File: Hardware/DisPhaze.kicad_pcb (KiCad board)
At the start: 2 copper layers, 71 x 24.1 mm, 13 parts, among them J1 Conn_01x27, J2 Conn_01x27, J3 Conn_01x04_Male, U1 STM32F405RGTx, Y1 Crystal

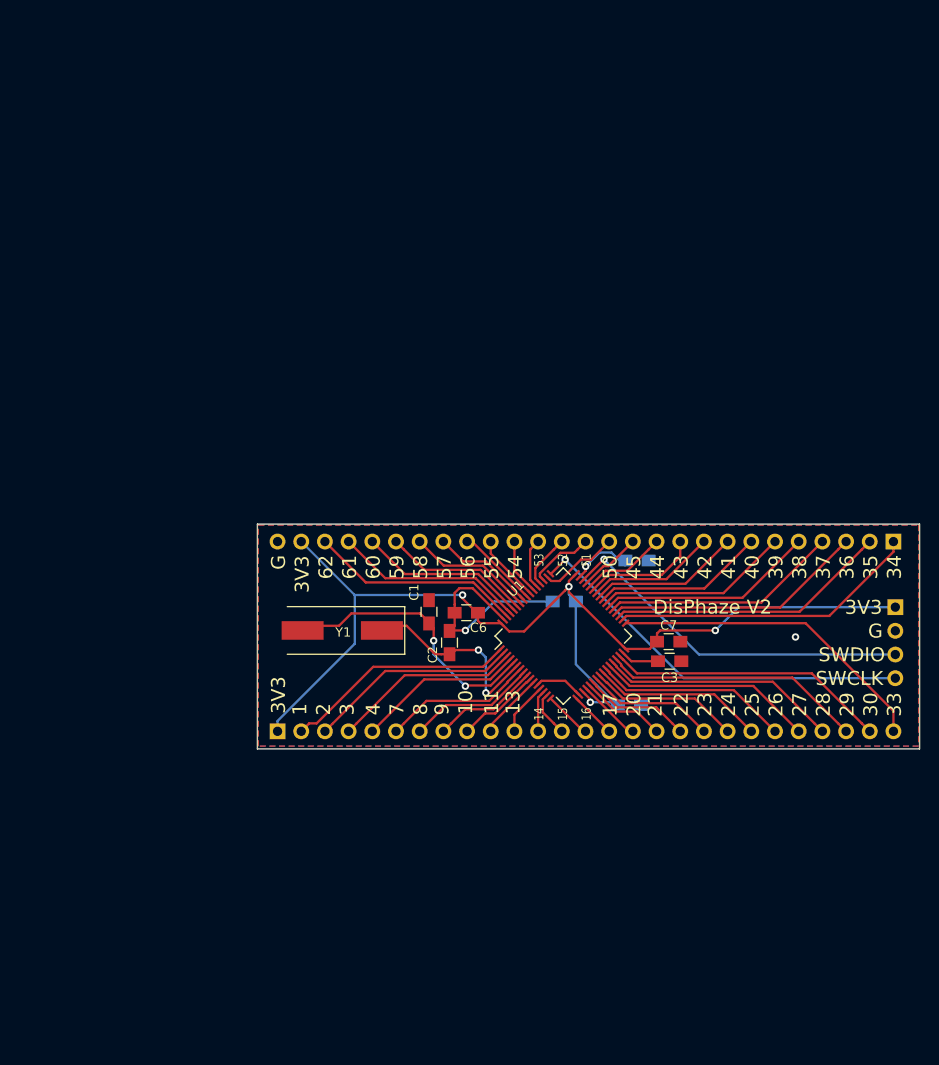
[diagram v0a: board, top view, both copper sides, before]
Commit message: Start PCB layout
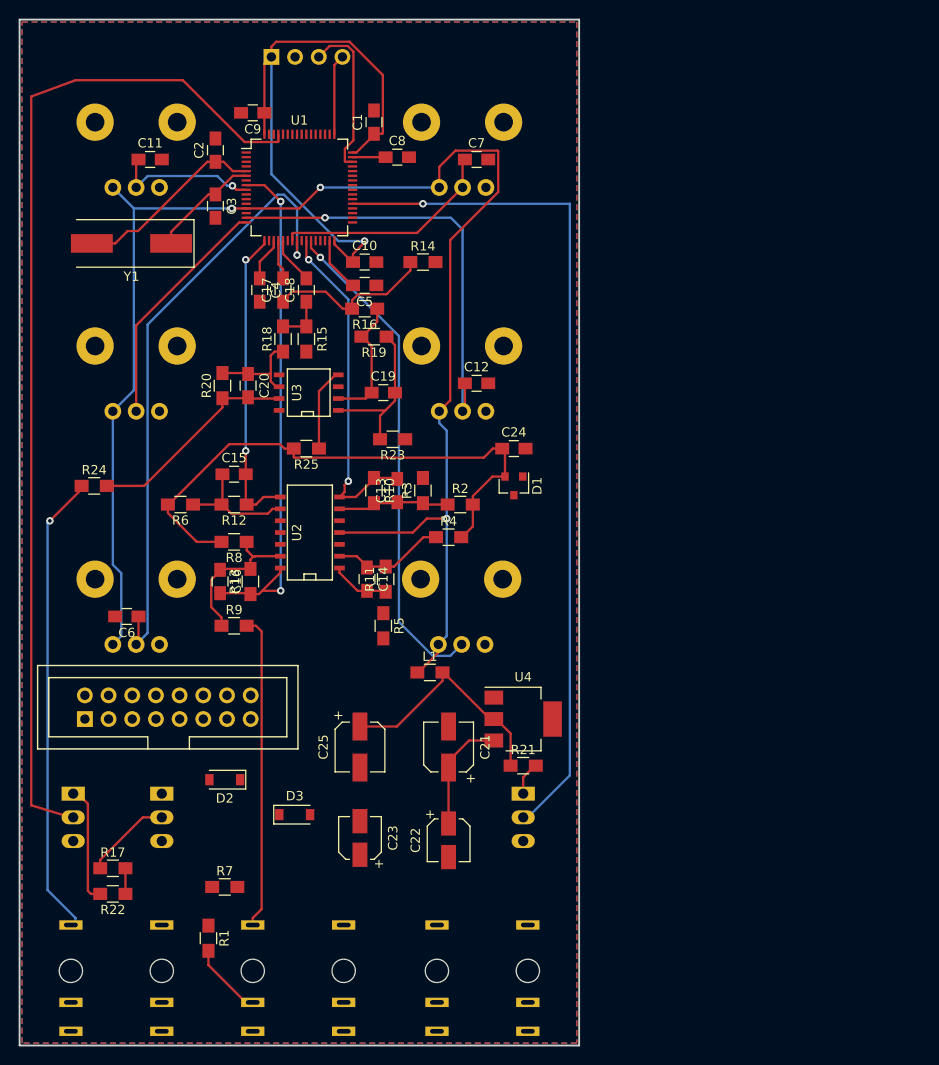
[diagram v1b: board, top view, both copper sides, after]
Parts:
- added C10: 100nF, Capacitors_SMD:C_0805_HandSoldering, F.Cu at (137.0, 76.0)
- added C11: 100nF, Capacitors_SMD:C_0805_HandSoldering, F.Cu at (114.0, 65.0)
- added C12: 100nF, Capacitors_SMD:C_0805_HandSoldering, F.Cu at (149.0, 89.0)
- added C13: 1nF, Capacitors_SMD:C_0805_HandSoldering, F.Cu at (140.5, 100.5)
- added C14: 2.2nF, Capacitors_SMD:C_0805_HandSoldering, F.Cu at (137.2, 110.0)
- added C15: 2.2nF, Capacitors_SMD:C_0805_HandSoldering, F.Cu at (123.0, 98.8)
- added C16: 1nF, Capacitors_SMD:C_0805_HandSoldering, F.Cu at (121.5, 110.2)
- added C17: 10uF, Capacitors_SMD:C_0805_HandSoldering, F.Cu at (128.2, 79.0)
- added C18: 10uF, Capacitors_SMD:C_0805_HandSoldering, F.Cu at (130.8, 79.0)
- added C19: 18pF, Capacitors_SMD:C_0805_HandSoldering, F.Cu at (139.0, 90.0)
- added C20: 18pF, Capacitors_SMD:C_0805_HandSoldering, F.Cu at (124.5, 89.2)
- added C21: 47uF, Capacitors_SMD:CP_Elec_5x5.8, F.Cu at (146.0, 128.0)
- added C22: 22uF, Capacitors_SMD:CP_Elec_4x5.8, F.Cu at (146.0, 138.0)
- added C23: 22uF, Capacitors_SMD:CP_Elec_4x5.8, F.Cu at (136.5, 137.8)
- added C24: 100nF, Capacitors_SMD:C_0805_HandSoldering, F.Cu at (153.0, 96.0)
- added C25: 47uF, Capacitors_SMD:CP_Elec_5x5.8, F.Cu at (136.5, 128.0)
- added C9: 100nF, Capacitors_SMD:C_0805_HandSoldering, F.Cu at (125.0, 60.0)
- added CTune1: B10k, Potentiometers:Potentiometer_Alps_RK09K_Horizontal, B.Cu at (144.9, 117.0)
- added D1: LM4040DBZ-5, TO_SOT_Packages_SMD:SOT-23, F.Cu at (153.0, 100.0)
- added D2: 1N5819, Diodes_SMD:D_SOD-123, F.Cu at (122.0, 131.5)
- added D3: 1N5819, Diodes_SMD:D_SOD-123, F.Cu at (129.5, 135.2)
- added FTune1: B10k, Potentiometers:Potentiometer_Alps_RK09K_Horizontal, B.Cu at (110.0, 117.0)
- added J4: PD2_Amt_In, Custom_Footprints:THONKICONN_hole, B.Cu at (115.2, 152.0)
- added J5: VCA_In, Custom_Footprints:THONKICONN_hole, B.Cu at (125.0, 152.0)
- added J6: DAC1_Out, Custom_Footprints:THONKICONN_hole, B.Cu at (154.5, 152.0)
- added J7: DAC2_Out, Custom_Footprints:THONKICONN_hole, B.Cu at (105.5, 152.0)
- added J8: Eurorack_16_pin_power, Custom_Footprints:Eurorack_16_pin_header, F.Cu at (107.0, 125.0)
- added L1: L, Resistors_SMD:R_0805_HandSoldering, F.Cu at (144.0, 120.0)
- added PD1Amt1: B10k, Potentiometers:Potentiometer_Alps_RK09K_Horizontal, B.Cu at (145.0, 68.0)
- added PD1Type1: B10k, Potentiometers:Potentiometer_Alps_RK09K_Horizontal, B.Cu at (145.0, 92.0)
- added PD2Amt1: B10k, Potentiometers:Potentiometer_Alps_RK09K_Horizontal, B.Cu at (110.0, 68.0)
- added PD2Type1: B10k, Potentiometers:Potentiometer_Alps_RK09K_Horizontal, B.Cu at (110.0, 92.0)
- added R1: 47k, Resistors_SMD:R_0805_HandSoldering, F.Cu at (120.2, 148.5)
- added R10: 47k, Resistors_SMD:R_0805_HandSoldering, F.Cu at (138.0, 100.5)
- added R11: 56k, Resistors_SMD:R_0805_HandSoldering, F.Cu at (139.2, 110.0)
- added R12: 47k, Resistors_SMD:R_0805_HandSoldering, F.Cu at (123.0, 102.0)
- added R13: 47k, Resistors_SMD:R_0805_HandSoldering, F.Cu at (124.8, 110.2)
- added R14: 47k, Resistors_SMD:R_0805_HandSoldering, F.Cu at (143.2, 76.0)
- added R15: 47k, Resistors_SMD:R_0805_HandSoldering, F.Cu at (130.8, 84.2)
- added R16: 6.3k, Resistors_SMD:R_0805_HandSoldering, F.Cu at (137.0, 81.0)
- added R17: 680R, Resistors_SMD:R_0805_HandSoldering, F.Cu at (110.0, 141.0)
- added R18: 6.3k, Resistors_SMD:R_0805_HandSoldering, F.Cu at (128.2, 84.2)
- added R19: 68k, Resistors_SMD:R_0805_HandSoldering, F.Cu at (138.0, 84.0)
- added R2: 82k, Resistors_SMD:R_0805_HandSoldering, F.Cu at (147.2, 102.0)
- added R20: 68k, Resistors_SMD:R_0805_HandSoldering, F.Cu at (121.8, 89.2)
- added R21: 680R, Resistors_SMD:R_0805_HandSoldering, F.Cu at (154.0, 130.0)
- added R22: 680R, Resistors_SMD:R_0805_HandSoldering, F.Cu at (110.0, 143.8)
- added R23: 1k, Resistors_SMD:R_0805_HandSoldering, F.Cu at (140.0, 95.0)
- added R24: 1k, Resistors_SMD:R_0805_HandSoldering, F.Cu at (108.0, 100.0)
- added R25: 2.2k, Resistors_SMD:R_0805_HandSoldering, F.Cu at (130.8, 96.0)
- added R3: 100k, Resistors_SMD:R_0805_HandSoldering, F.Cu at (143.2, 100.5)
- added R4: 91k, Resistors_SMD:R_0805_HandSoldering, F.Cu at (146.0, 105.5)
- added R5: 100k, Resistors_SMD:R_0805_HandSoldering, F.Cu at (139.0, 115.0)
- added R6: 68k, Resistors_SMD:R_0805_HandSoldering, F.Cu at (117.2, 102.0)
- added R7: 100k, Resistors_SMD:R_0805_HandSoldering, F.Cu at (122.0, 143.0)
- added R8: 68k, Resistors_SMD:R_0805_HandSoldering, F.Cu at (123.0, 106.0)
- added R9: 100k, Resistors_SMD:R_0805_HandSoldering, F.Cu at (123.0, 115.0)
- added SW1: DAC1_RingMod_Switch, Custom_Footprints:SPDTSubMiniature, B.Cu at (154.0, 133.0)
- added SW2: DAC2_Mix_Switch, Custom_Footprints:SPDTSubMiniature, B.Cu at (105.8, 133.0)
- added SW3: Octave_Switch, Custom_Footprints:SPDTSubMiniature, B.Cu at (115.2, 133.0)
- added U2: MCP6004, SMD_Packages:SOIC-14_N, F.Cu at (131.0, 105.0)
- added U3: TL072, SMD_Packages:SOIC-8-N, F.Cu at (131.0, 90.0)
- added U4: LM1117-3.3, TO_SOT_Packages_SMD:SOT-223, F.Cu at (154.0, 125.0)
- C1: value 18pF -> 100nF
- C3: value 2.2uF -> 18pF
- C4: value 2.2uF -> 100nF; moved to F.Cu
- C5, C8: value 100nF -> 2.2uF; moved to F.Cu
- J1: value Conn_01x27 -> SWD_Header; footprint Custom_Footprints:Connector_27x2.54mm -> Custom_Footprints:4pin_header
- J2: value Conn_01x27 -> PItch_In; footprint Custom_Footprints:Connector_27x2.54mm -> Custom_Footprints:THONKICONN_hole; moved to B.Cu
- J3: value Conn_01x04_Male -> PD1_Amt_In; footprint Custom_Footprints:4pin_header -> Custom_Footprints:THONKICONN_hole; moved to B.Cu
- moved J2 74.8 mm to (134.8, 152.0)
- moved J1 72.3 mm to (127.0, 54.0)
- moved C3 68.9 mm to (121.0, 70.0), turned to 270 degrees
- moved C8 63.8 mm to (140.5, 64.8)
- moved J3 62.7 mm to (144.8, 152.0), turned to 180 degrees
- moved C2 58.5 mm to (121.0, 64.0)
- moved U1 55.8 mm to (130.0, 68.0), turned to 0 degrees
- moved C7 55.7 mm to (149.0, 65.0)
- moved C1 52.8 mm to (138.0, 61.0)
- moved C4 49.8 mm to (125.8, 79.0), turned to 270 degrees
- moved Y1 47.3 mm to (112.0, 74.0)
- moved C5 40.1 mm to (137.0, 78.5)
- moved C6 36.4 mm to (111.5, 114.0)
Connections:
- C1 pad 1: Net-(C1-Pad1) -> +3V3
- C3 pad 1: GND -> Net-(C3-Pad1)
- C3 pad 2: Net-(C3-Pad2) -> GND
- C4 pad 1: Net-(C4-Pad1) -> +3V3
- C5 pad 1: +3V3 -> GND
- C5 pad 2: GND -> Net-(C5-Pad2)
- C6 pad 1: +3V3 -> FTUNE
- C7 pad 1: +3V3 -> PD1_POT
- C8 pad 1: +3V3 -> Net-(C8-Pad1)
- J1 pad 2: p1 -> GND
- J1 pad 3: p2 -> SWDIO
- J1 pad 4: p3 -> SWCLK
- J2 pad 1: p34 -> GND
- J2 pad 2: p35 -> CV_IN
- J2 pad 3: p36 -> Net-(J2-Pad3)
- J3 pad 1: +3V3 -> GND
- J3 pad 3: SWDIO -> Net-(J3-Pad3)
- U1 pad 1: p1 -> Net-(U1-Pad1)
- U1 pad 10: p10 -> PD1_CV
- U1 pad 11: p11 -> Net-(U1-Pad11)
- U1 pad 13: p13 -> +3.3VA
- U1 pad 14: p14 -> Net-(U1-Pad14)
- U1 pad 15: p15 -> PD1_TYPE
- U1 pad 16: p16 -> PD2_TYPE
- U1 pad 17: p17 -> PD2_CV
- U1 pad 2: p2 -> Net-(U1-Pad2)
- U1 pad 20: p20 -> DAC1_OUT
- U1 pad 21: p21 -> DAC2_OUT
- U1 pad 22: p22 -> Net-(U1-Pad22)
- U1 pad 23: p23 -> PD1_POT
- U1 pad 24: p24 -> FTUNE
- U1 pad 25: p25 -> Net-(U1-Pad25)
- U1 pad 26: p26 -> V_OCT_CV
- U1 pad 27: p27 -> CTUNE
- U1 pad 28: p28 -> Net-(U1-Pad28)
- U1 pad 29: p29 -> Net-(U1-Pad29)
- U1 pad 3: p3 -> Net-(U1-Pad3)
- U1 pad 30: p30 -> Net-(U1-Pad30)
- U1 pad 31: Net-(C3-Pad2) -> Net-(C5-Pad2)
- U1 pad 33: p33 -> OCTAVE_UP
- U1 pad 34: p34 -> OCTAVE_DN
- U1 pad 35: p35 -> Net-(U1-Pad35)
- U1 pad 36: p36 -> Net-(U1-Pad36)
- U1 pad 37: p37 -> DAC1_RING_MOD
- U1 pad 38: p38 -> Net-(U1-Pad38)
- U1 pad 39: p39 -> Net-(U1-Pad39)
- U1 pad 4: p4 -> Net-(U1-Pad4)
- U1 pad 40: p40 -> Net-(U1-Pad40)
- U1 pad 41: p41 -> Net-(U1-Pad41)
- U1 pad 42: p42 -> Net-(U1-Pad42)
- U1 pad 43: p43 -> Net-(U1-Pad43)
- U1 pad 44: p44 -> Net-(U1-Pad44)
- U1 pad 45: p45 -> Net-(U1-Pad45)
- U1 pad 47: Net-(C4-Pad1) -> Net-(C8-Pad1)
- U1 pad 5: Net-(C1-Pad1) -> Net-(C2-Pad1)
- U1 pad 50: p50 -> Net-(U1-Pad50)
- U1 pad 51: p51 -> Net-(U1-Pad51)
- U1 pad 52: p52 -> Net-(U1-Pad52)
- U1 pad 53: p53 -> Net-(U1-Pad53)
- U1 pad 54: p54 -> Net-(U1-Pad54)
- U1 pad 55: p55 -> Net-(U1-Pad55)
- U1 pad 56: p56 -> Net-(U1-Pad56)
- U1 pad 57: p57 -> Net-(U1-Pad57)
- U1 pad 58: p58 -> Net-(U1-Pad58)
- U1 pad 59: p59 -> Net-(U1-Pad59)
- U1 pad 6: Net-(C2-Pad1) -> Net-(C3-Pad1)
- U1 pad 60: p60 -> Net-(U1-Pad60)
- U1 pad 61: p61 -> DAC2_MIX
- U1 pad 62: p62 -> Net-(U1-Pad62)
- U1 pad 7: p7 -> Net-(U1-Pad7)
- U1 pad 8: p8 -> VCA
- U1 pad 9: p9 -> PD2_POT
- Y1 pad 1: Net-(C2-Pad1) -> Net-(C3-Pad1)
- Y1 pad 2: Net-(C1-Pad1) -> Net-(C2-Pad1)
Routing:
- net +3.3VA: track 0.00 -> 166.9 mm, vias 0 -> 3
- net DAC2_MIX: track 0.00 -> 111.3 mm
- net DAC1_RING_MOD: track 0.00 -> 91.5 mm, vias 0 -> 1
- net FTUNE: track 0.00 -> 66.9 mm, vias 0 -> 1
- net AREF_-5: track 0.00 -> 60.4 mm
- net VCA: track 0.00 -> 56.1 mm, vias 0 -> 2
- net CTUNE: track 0.00 -> 53.5 mm, vias 0 -> 1
- net Net-(J7-Pad3): track 0.00 -> 49.8 mm, vias 0 -> 1
- net PD1_TYPE: track 0.00 -> 46.3 mm, vias 0 -> 1
- net V_OCT_CV: track 0.00 -> 36.9 mm, vias 0 -> 2
- net p33: track 34.8 -> 0.00 mm
- net SWCLK: track 42.9 -> 8.66 mm, vias 1 -> 0
- net Net-(J5-Pad3): track 0.00 -> 33.7 mm
- net PD2_CV: track 0.00 -> 33.3 mm, vias 0 -> 2
- net p34: track 33.2 -> 0.00 mm
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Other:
- board size 71 x 24.1 mm -> 60 x 110 mm
- rule pad_to_mask_clearance: 0.051 -> 0
- board text removed: "1"
- board text removed: "10"
- board text removed: "11"
- board text removed: "13"
- board text removed: "14"
- board text removed: "15"
- board text removed: "16"
- board text removed: "17"
- board text removed: "2"
- board text removed: "20"
- board text removed: "21"
- board text removed: "22"
- board text removed: "23"
- board text removed: "24"
- board text removed: "25"
- board text removed: "26"
- board text removed: "27"
- board text removed: "28"
- board text removed: "29"
- board text removed: "3"
- board text removed: "30"
- board text removed: "33"
- board text removed: "34"
- board text removed: "35"
- board text removed: "36"
- board text removed: "37"
- board text removed: "38"
- board text removed: "39"
- board text removed: "3V3"
- board text removed: "4"
- board text removed: "40"
- board text removed: "41"
- board text removed: "42"
- board text removed: "43"
- board text removed: "44"
- board text removed: "45"
- board text removed: "50"
- board text removed: "51"
- board text removed: "52"
- board text removed: "53"
- board text removed: "54"
- board text removed: "55"
- board text removed: "56"
- board text removed: "57"
- board text removed: "58"
- board text removed: "59"
- board text removed: "60"
- board text removed: "61"
- board text removed: "62"
- board text removed: "7"
- board text removed: "8"
- board text removed: "9"
- board text removed: "DisPhaze V2"
- board text removed: "G"
- board text removed: "SWCLK"
- board text removed: "SWDIO"
